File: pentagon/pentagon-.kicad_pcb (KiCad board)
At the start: 2 copper layers, 80.9 x 76.9 mm, 28 parts, among them J1 Conn_01x05_Pin, J2 Conn_01x05_Pin, J3 Conn_01x05_Pin, J4 Conn_01x05_Pin, J5 Conn_01x05_Pin

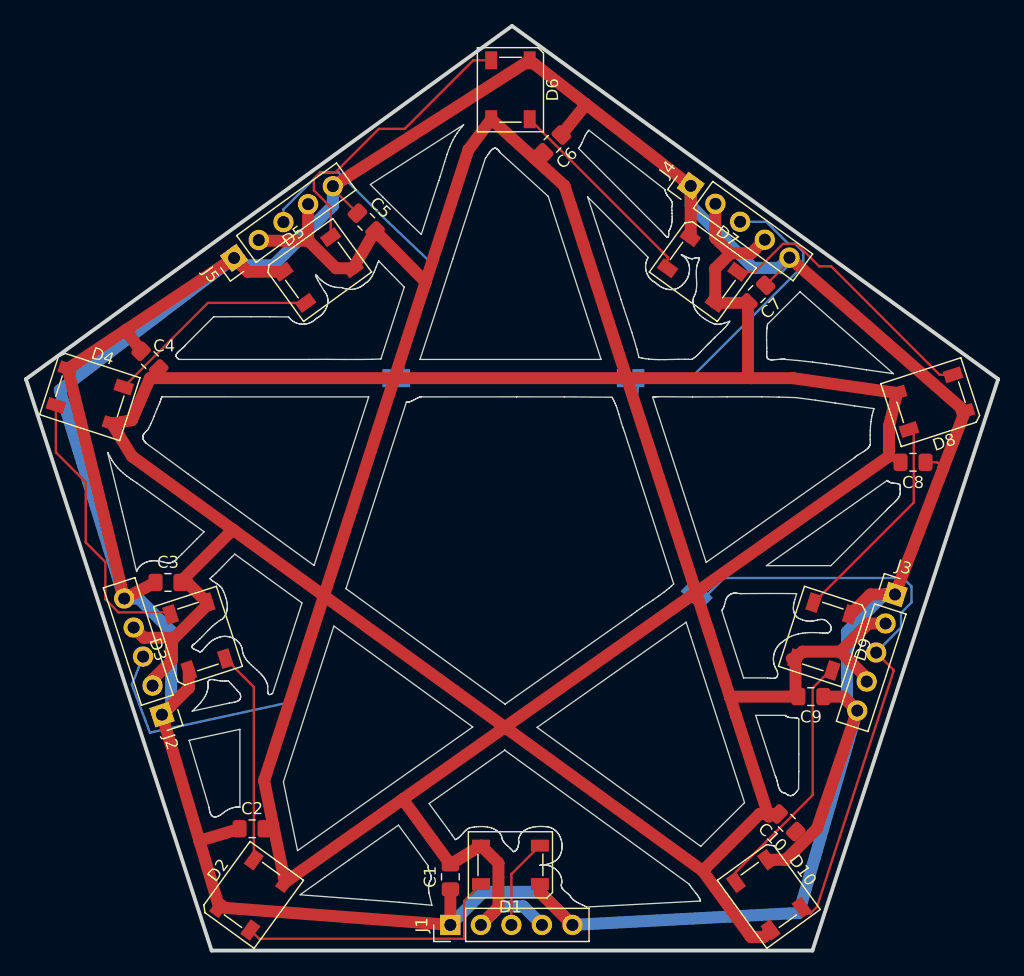
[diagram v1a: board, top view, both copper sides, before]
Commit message: updated all coolness
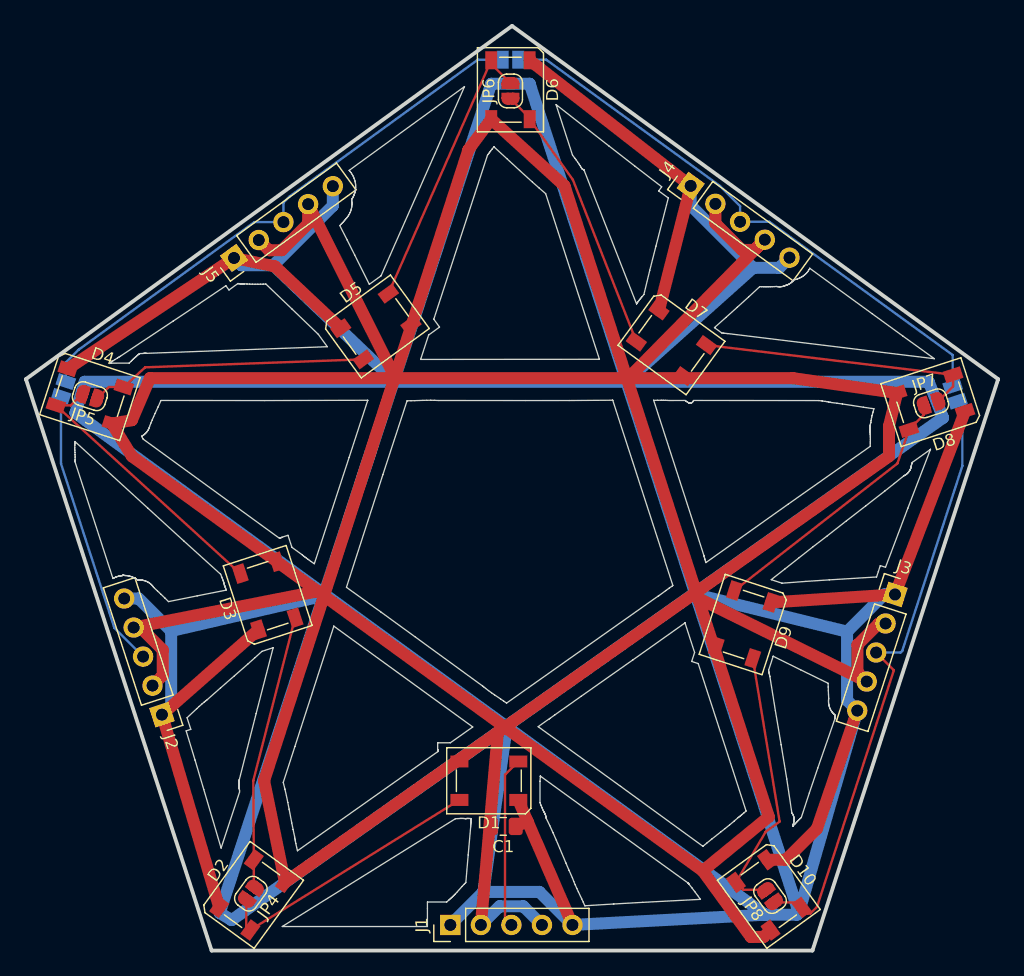
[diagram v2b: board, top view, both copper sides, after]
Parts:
- removed C10, C2, C3, C4, C5, C6, C7, C8, C9: C, Capacitor_SMD:C_0805_2012Metric_Pad1.18x1.45mm_HandSolder
- added JP4: SolderJumper_2_Open, Jumper:SolderJumper-2_P1.3mm_Open_RoundedPad1.0x1.5mm, F.Cu at (78.4, 95.4)
- added JP5: SolderJumper_2_Open, Jumper:SolderJumper-2_P1.3mm_Open_RoundedPad1.0x1.5mm, F.Cu at (65.0, 54.0)
- added JP6: SolderJumper_2_Open, Jumper:SolderJumper-2_P1.3mm_Open_RoundedPad1.0x1.5mm, F.Cu at (100.0, 28.6)
- added JP7: SolderJumper_2_Open, Jumper:SolderJumper-2_P1.3mm_Open_RoundedPad1.0x1.5mm, F.Cu at (135.0, 54.6)
- added JP8: SolderJumper_2_Open, Jumper:SolderJumper-2_P1.3mm_Open_RoundedPad1.0x1.5mm, F.Cu at (121.6, 95.6)
- moved JP3 28.3 mm to (100.0, 26.0)
- moved JP2 27.7 mm to (62.8, 53.4), turned to 72 degrees
- moved JP1 27.2 mm to (137.0, 53.8), turned to -72 degrees
- moved D1 7.23 mm to (98.2, 86.0)
- moved D3 6.72 mm to (79.8, 70.6)
- moved D5 6.72 mm to (88.8, 48.2)
- moved D9 6.68 mm to (119.4, 73.0)
- moved D7 6.63 mm to (113.4, 49.6)
- moved C1 6.08 mm to (99.4, 89.8), turned to 180 degrees
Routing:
- net GND: track 342.7 -> 672.9 mm
- net Net-(J2-Pin_3): track 46.9 -> 23.3 mm
- net Net-(D1-DIN): track 7.58 -> 14.3 mm
- net Net-(D6-DOUT): track 17.2 -> 23.0 mm
- net Net-(D2-DOUT): track 17.7 -> 22.9 mm
- net Net-(D4-DOUT): track 18.0 -> 23.2 mm
- net Net-(D8-DOUT): track 18.0 -> 22.7 mm
- net Net-(J4-Pin_3): track 43.2 -> 47.8 mm
- net Net-(D10-DIN): track 21.0 -> 22.8 mm
- net Net-(J5-Pin_3): track 45.9 -> 47.4 mm
- net Net-(D10-DOUT): track 49.7 -> 50.9 mm
- net +5V: track 455.0 -> 455.7 mm
- net Net-(D3-DOUT): track 23.9 -> 23.4 mm
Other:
- outline, holes or cut-outs redrawn
